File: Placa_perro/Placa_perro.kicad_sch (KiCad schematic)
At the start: 48 parts, among them J1 S_TEMPERATURA, J10 TEST_POINT1, J11 PANTALLA, J12 ENTRADA, J14 SALIDA_3.3v, J15 ADC, J16 12v, J17 5v, J18 3.3v, J19 GND, J2 LDR, J20 LDR, J21 ADC, J22 SALIDA_RELE_1, J4 S_GAS1, J5 S_GAS2, J6 USB_B, J8 SALIDA_3.3v, J9 SALIDA_RELÉ, K2 Relay_SPDT, Q2 BC337, SW10 SW_Push, SW11 SW_Push, SW12 SW_Push, SW13 SW_Push, SW9 SW_Push, U2 LM7805_TO220

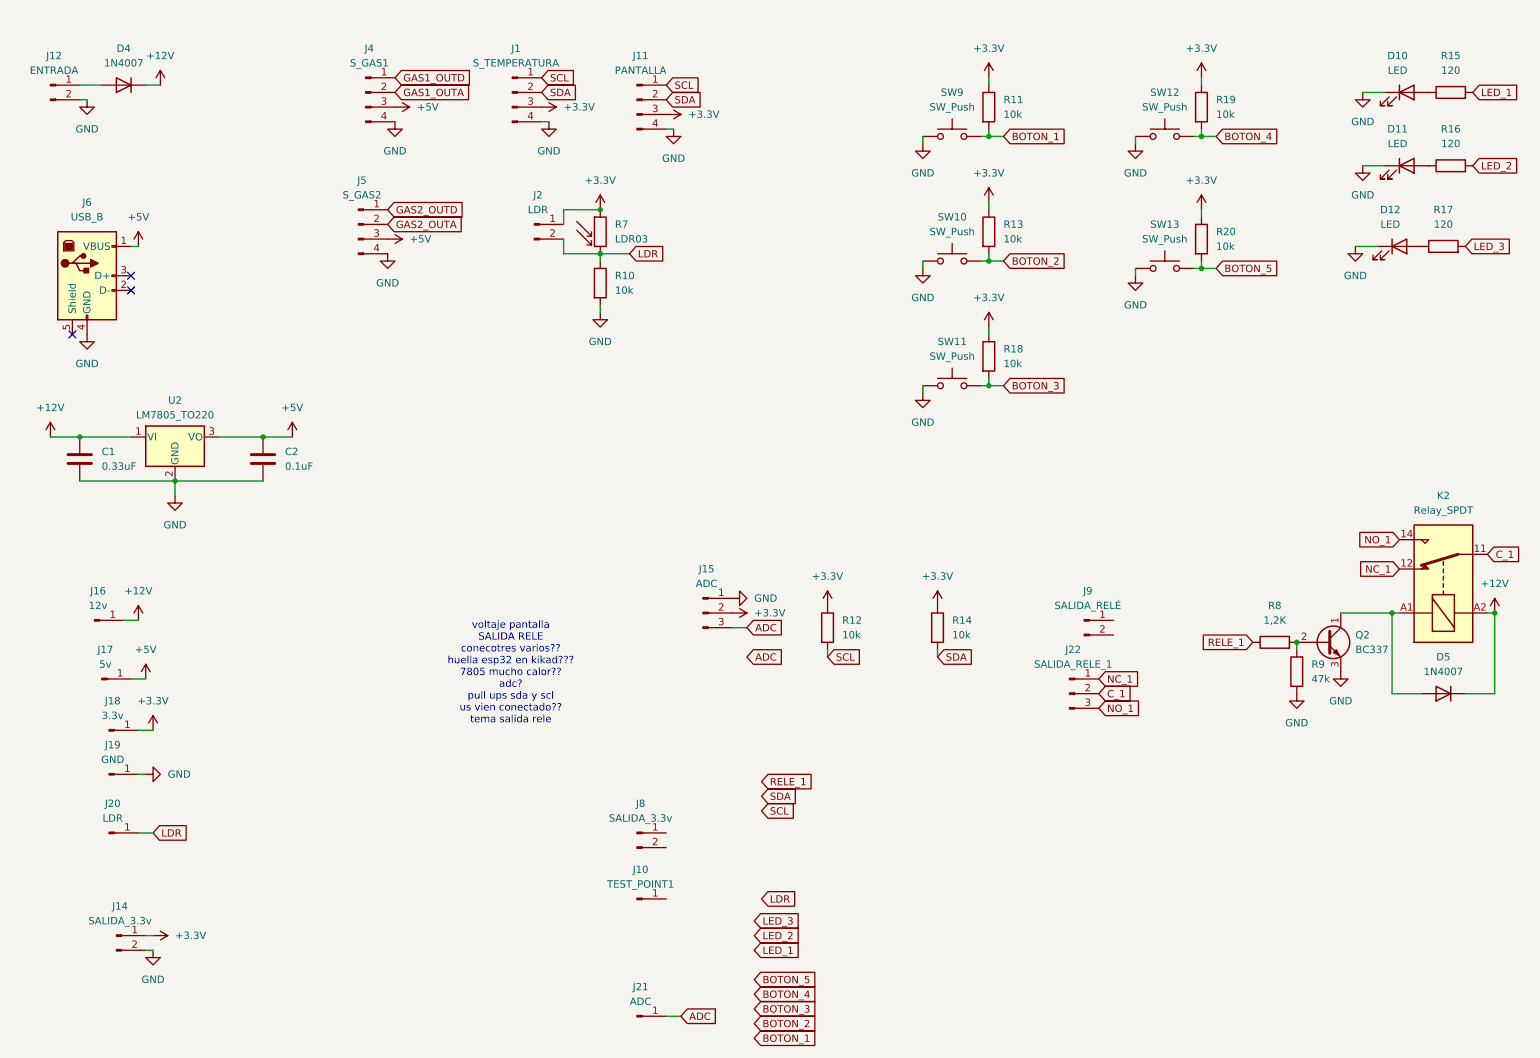
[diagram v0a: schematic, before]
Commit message: esq
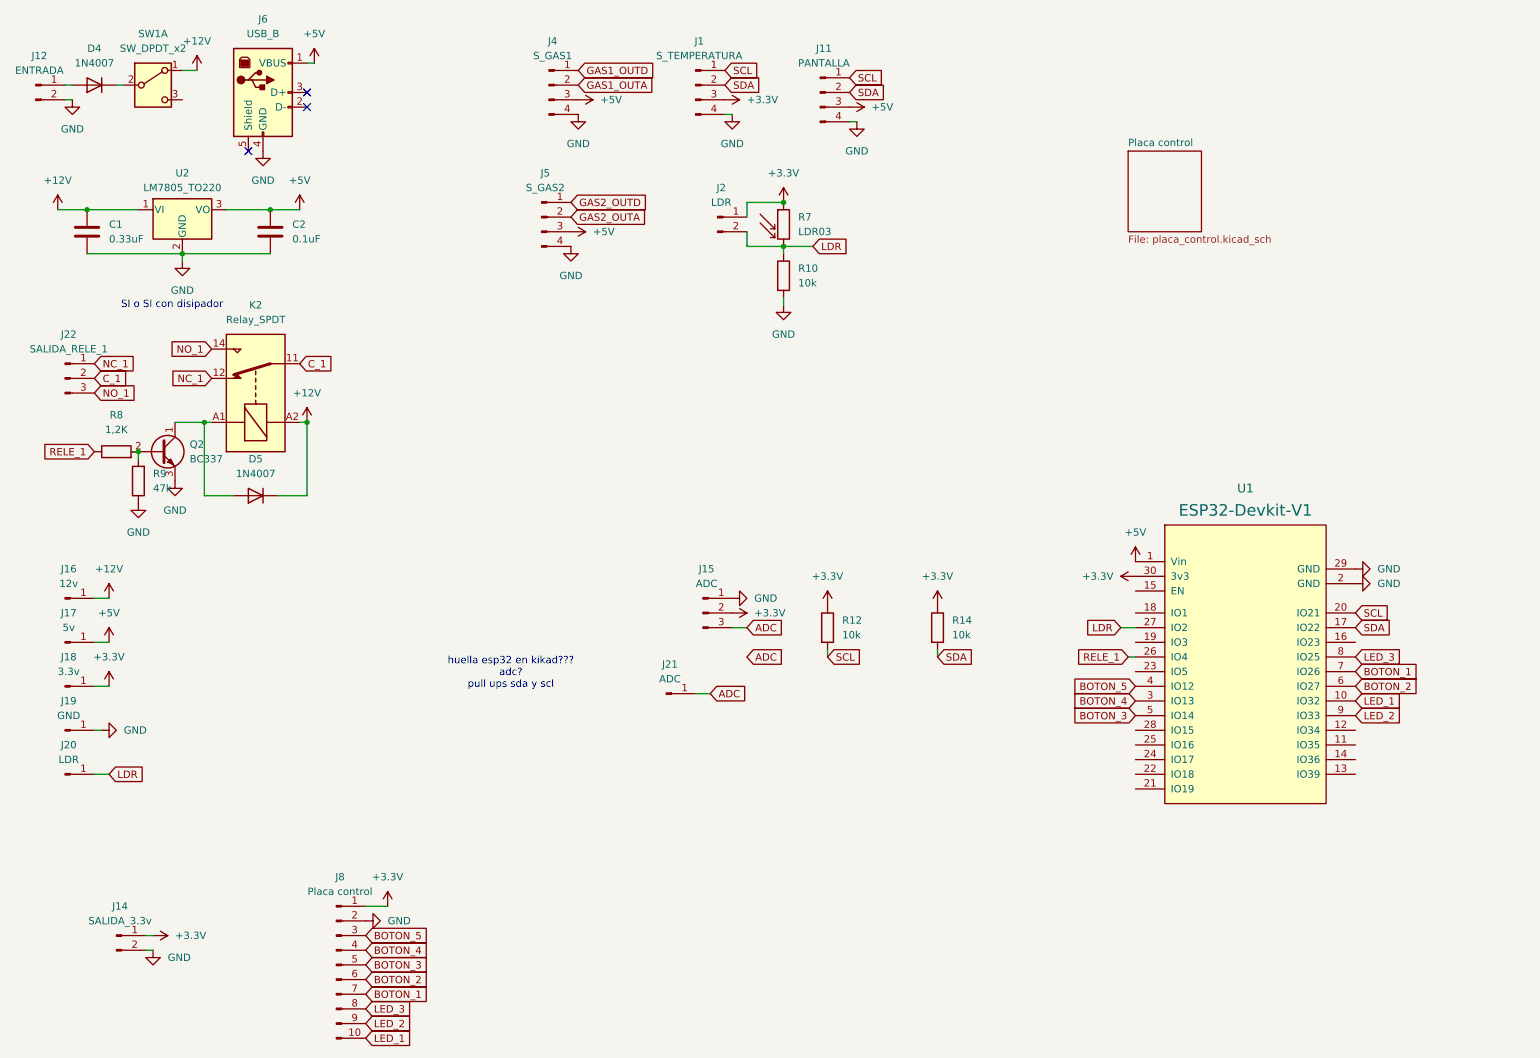
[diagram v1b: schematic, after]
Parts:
- removed D10, D11, D12: LED, LED_THT:LED_D3.0mm_Clear, symbol Device:LED
- removed J10: TEST_POINT1, symbol Connector:Conn_01x01_Pin
- removed J8: SALIDA_3.3v, symbol Connector:Conn_01x02_Pin
- removed J9: SALIDA_RELÉ, symbol Connector:Conn_01x02_Pin
- removed R11, R13, R18, R19, R20: 10k, Resistor_THT:R_Axial_DIN0207_L6.3mm_D2.5mm_P7.62mm_Horizontal, symbol Device:R
- removed R15, R16, R17: 120, Resistor_THT:R_Axial_DIN0207_L6.3mm_D2.5mm_P7.62mm_Horizontal, symbol Device:R
- removed SW10, SW11, SW12, SW13, SW9: SW_Push, Button_Switch_THT:SW_PUSH_6mm, symbol Switch:SW_Push
- added J8: Placa control, symbol Connector:Conn_01x10_Pin
- added SW1: SW_DPDT_x2, symbol Switch:SW_DPDT_x2
- added U1: ESP32-Devkit-V1, DOIT_ESP32:DOIT_ESP32_Devkit_mirko, symbol esp32-devkit-v1:ESP32-Devkit-V1
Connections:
- net +12V: now also SW1.1 (A); no longer D4.1 (K)
- net +3.3V: now also J8.1 (Pin_1), U1.30 (3v3); no longer J11.3 (Pin_3)
- net +5V: now also J11.3 (Pin_3), U1.1 (Vin)
- net BOTON_1: now also J8.7 (Pin_7), U1.7 (IO26)
- net BOTON_2: now also J8.6 (Pin_6), U1.6 (IO27)
- net BOTON_3: now also J8.5 (Pin_5), U1.5 (IO14)
- net BOTON_4: now also J8.4 (Pin_4), U1.3 (IO13)
- net BOTON_5: now also J8.3 (Pin_3), U1.4 (IO12)
- net GND: now also J8.2 (Pin_2), U1.2 (GND), U1.29 (GND)
- net LDR: now also U1.27 (IO2)
- net LED_1: now also J8.10 (Pin_10), U1.10 (IO32)
- net LED_2: now also J8.9 (Pin_9), U1.9 (IO33)
- net LED_3: now also J8.8 (Pin_8), U1.8 (IO25)
- net RELE_1: now also U1.26 (IO4)
- net SCL: now also U1.20 (IO21)
- net SDA: now also U1.17 (IO22)
- new net: D4.1 (K), SW1.2 (B)
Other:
- added sheet Placa control (placa_control.kicad_sch)
- note added: "SI o SI con disipador"
- note added: "huella esp32 en kikad??? adc? pull ups sda y scl"
- note removed: "voltaje pantalla SALIDA RELE conecotres varios?? huella esp32 en kikad??? 7805 mucho calor?? adc? pull ups sda y scl us vien conectado?? tema salida rele"
- moved on the sheet: C1, C2, D4, D5, J1, J11, J12, J16, J17, J18, J19, J2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
